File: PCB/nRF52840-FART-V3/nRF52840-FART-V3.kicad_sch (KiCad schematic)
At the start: 7 parts, among them U1 xiao-ble

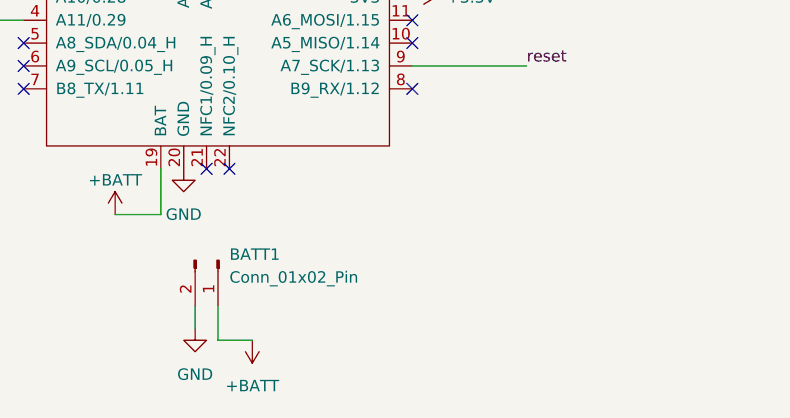
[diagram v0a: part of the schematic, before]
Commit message: Tweaks to the PCB design
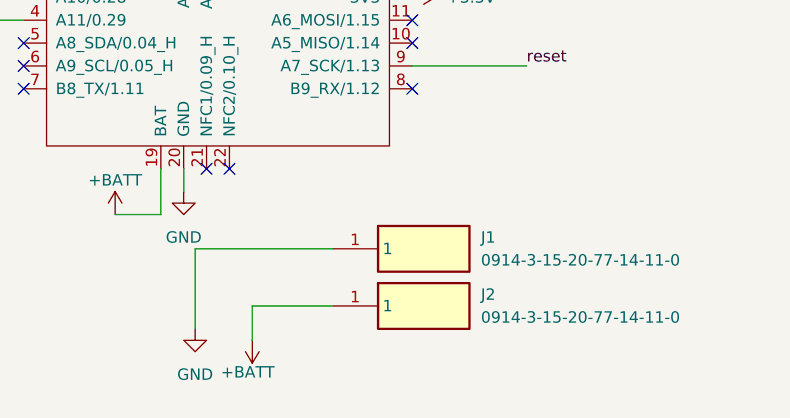
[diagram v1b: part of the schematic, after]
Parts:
- removed BATT1: Conn_01x02_Pin, Connector_JST:JST_PH_S2B-PH-K_1x02_P2.00mm_Horizontal, symbol Connector:Conn_01x02_Pin
- added J1, J2: 0914-3-15-20-77-14-11-0, 0914315207714110, symbol Samac:0914-3-15-20-77-14-11-0
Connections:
- net +BATT: now also J2.1
- net GND: now also J1.1
